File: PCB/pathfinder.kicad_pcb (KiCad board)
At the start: 2 copper layers, 150 x 100 mm, 18 parts, among them SW1 SW_Push, SW2 SW_Push, SW3 SW_Push, SW4 SW_Push, SW5 SW_Push, SW6 SW_Push, SW7 SW_Push, SW8 SW_Push, SW9 SW_Push, U2 XIAO-RP2040-DIP

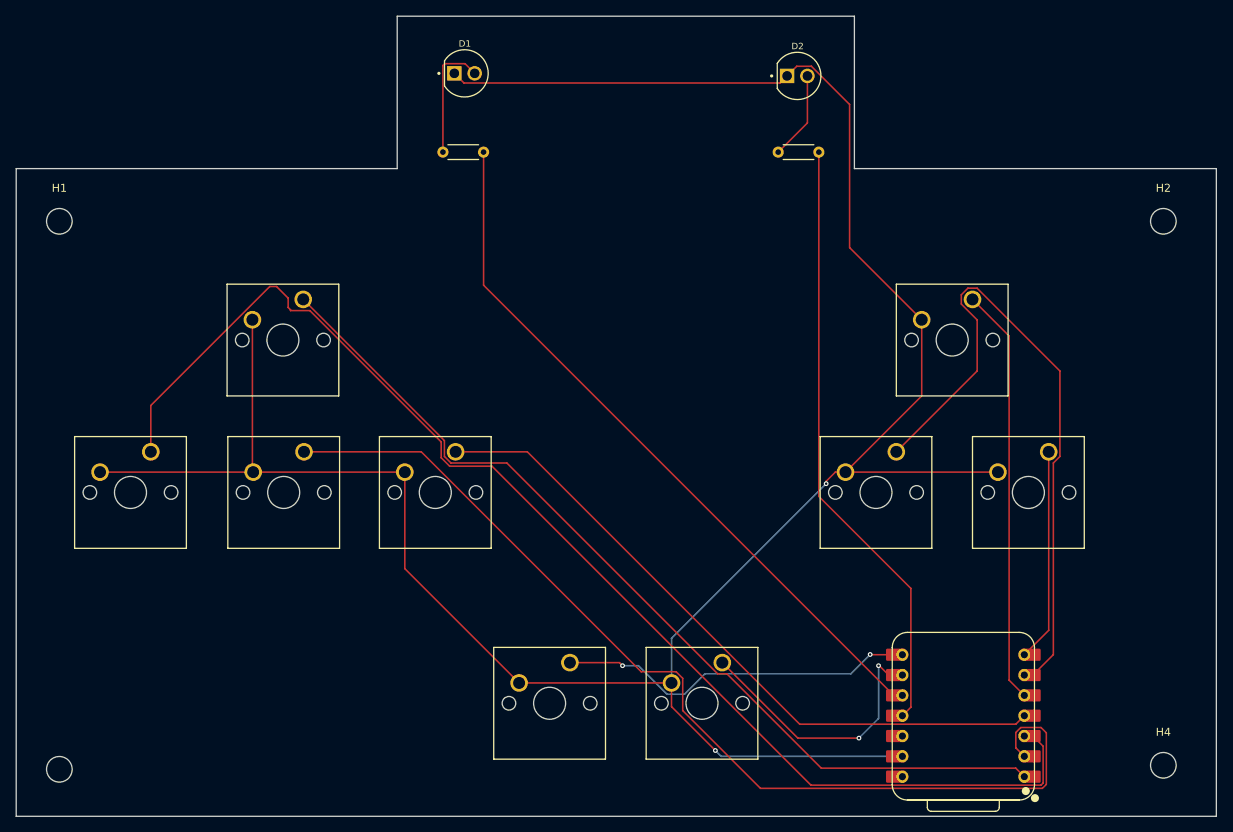
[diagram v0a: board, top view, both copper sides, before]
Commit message: gerber and pcb
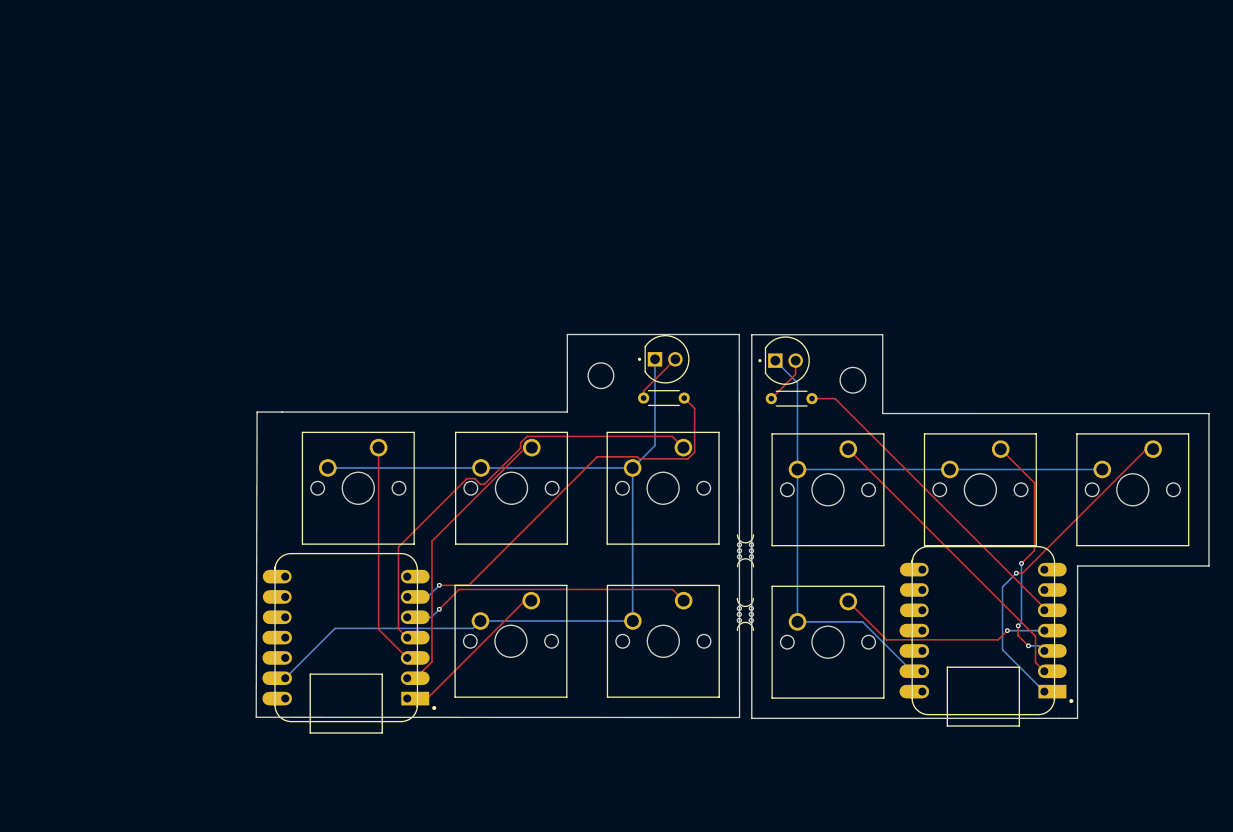
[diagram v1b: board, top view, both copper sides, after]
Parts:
- removed H1, H3: MountingHole, MountingHole:MountingHole_3.2mm_M3
- added HSMALL1: MountingHole, custom_footprints:mouse-bite-2mm-slot, F.Cu at (179.2, 117.6)
- added HSMALL2: MountingHole, custom_footprints:mouse-bite-2mm-slot, F.Cu at (179.3, 109.7)
- added U3: XIAO-RP2040-DIP, footprints:XIAO-Generic-Hybrid-14P-2.54-21X17.8MM, F.Cu at (209.0, 119.7)
- D1: value L08R5000Q1 -> POWER
- D2: value L08R5000Q1 -> Drift
- SW1: value SW_Push -> GAS
- SW2: value SW_Push -> BRAKE
- SW3: value SW_Push -> LEFT
- SW4: value SW_Push -> RIGHT
- SW5: value SW_Push -> CHECKPOINT
- SW6: value SW_Push -> RESTART
- SW7: value SW_Push -> AK40
- SW8: value SW_Push -> AK60
- SW9: value SW_Push -> AK80
- U2: footprint mito-keyboard mito-simplified main Seeed Studio XIAO Series Library:XIAO-RP2040-DIP -> footprints:XIAO-Generic-Hybrid-14P-2.54-21X17.8MM
- moved U2 77.8 mm to (129.4, 120.5)
- moved HBIG1 72.9 mm to (161.2, 87.8)
- moved HBIG2 61.8 mm to (192.7, 88.4)
- moved SW1 47.2 mm to (152.5, 115.9)
- moved D1 43.7 mm to (169.2, 85.8)
- moved R1 39.7 mm to (166.5, 90.6)
- moved D2 35.6 mm to (184.3, 85.9)
- moved R2 30.8 mm to (182.5, 90.7)
- moved SW5 29.3 mm to (230.2, 97.0)
- moved SW2 28.5 mm to (152.6, 96.8)
- moved SW3 28.5 mm to (133.4, 96.8)
- moved SW4 28.5 mm to (171.5, 96.8)
- moved SW9 17.5 mm to (192.1, 116.0)
- moved SW8 16.2 mm to (171.5, 115.9)
- moved SW6 6.01 mm to (192.1, 97.0)
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- renumbered H2 to HBIG1, H4 to HBIG2
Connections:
- U2 pad 10: POWER -> unconnected-(U2-GPIO4/MISO-Pad10)
- U2 pad 11: Drift Indicator -> unconnected-(U2-GPIO3/MOSI-Pad11)
- U2 pad 5: CHECKPOINT -> AK60
- U2 pad 6: RESTART -> POWER
- U2 pad 7: AK40 -> unconnected-(U2-GPIO0/TX-Pad7)
- U2 pad 8: AK60 -> unconnected-(U2-GPIO1/RX-Pad8)
- U2 pad 9: AK80 -> unconnected-(U2-GPIO2/SCK-Pad9)
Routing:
- net LEFT: track 158.8 -> 27.8 mm
- net GND: track 304.5 -> 208.5 mm, vias 2 -> 0
- net GAS: track 116.0 -> 20.6 mm
- net BRAKE: track 127.0 -> 36.3 mm
- net RESTART: track 82.1 -> 37.9 mm
- net POWER: track 90.2 -> 50.9 mm, vias 0 -> 1
- net Drift Indicator: track 75.7 -> 40.2 mm
- net RIGHT: track 85.6 -> 54.7 mm
- net CHECKPOINT: track 52.2 -> 42.2 mm, vias 0 -> 1
- net Net-(D1-PadA): track 15.4 -> 6.49 mm
- net AK60: track 45.3 -> 36.6 mm, vias 2 -> 1
- net AK80: track 34.5 -> 27.0 mm, vias 2 -> 1
- net Net-(D2-PadA): track 11.0 -> 6.01 mm
- net AK40: track 26.6 -> 31.4 mm, vias 0 -> 3
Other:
- board size 150 x 100 mm -> 119.1 x 48 mm
